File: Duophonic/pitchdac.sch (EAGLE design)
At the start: 30 parts, among them IC1 AD5781ARUZ, U1 opa2186, U2 opa2186

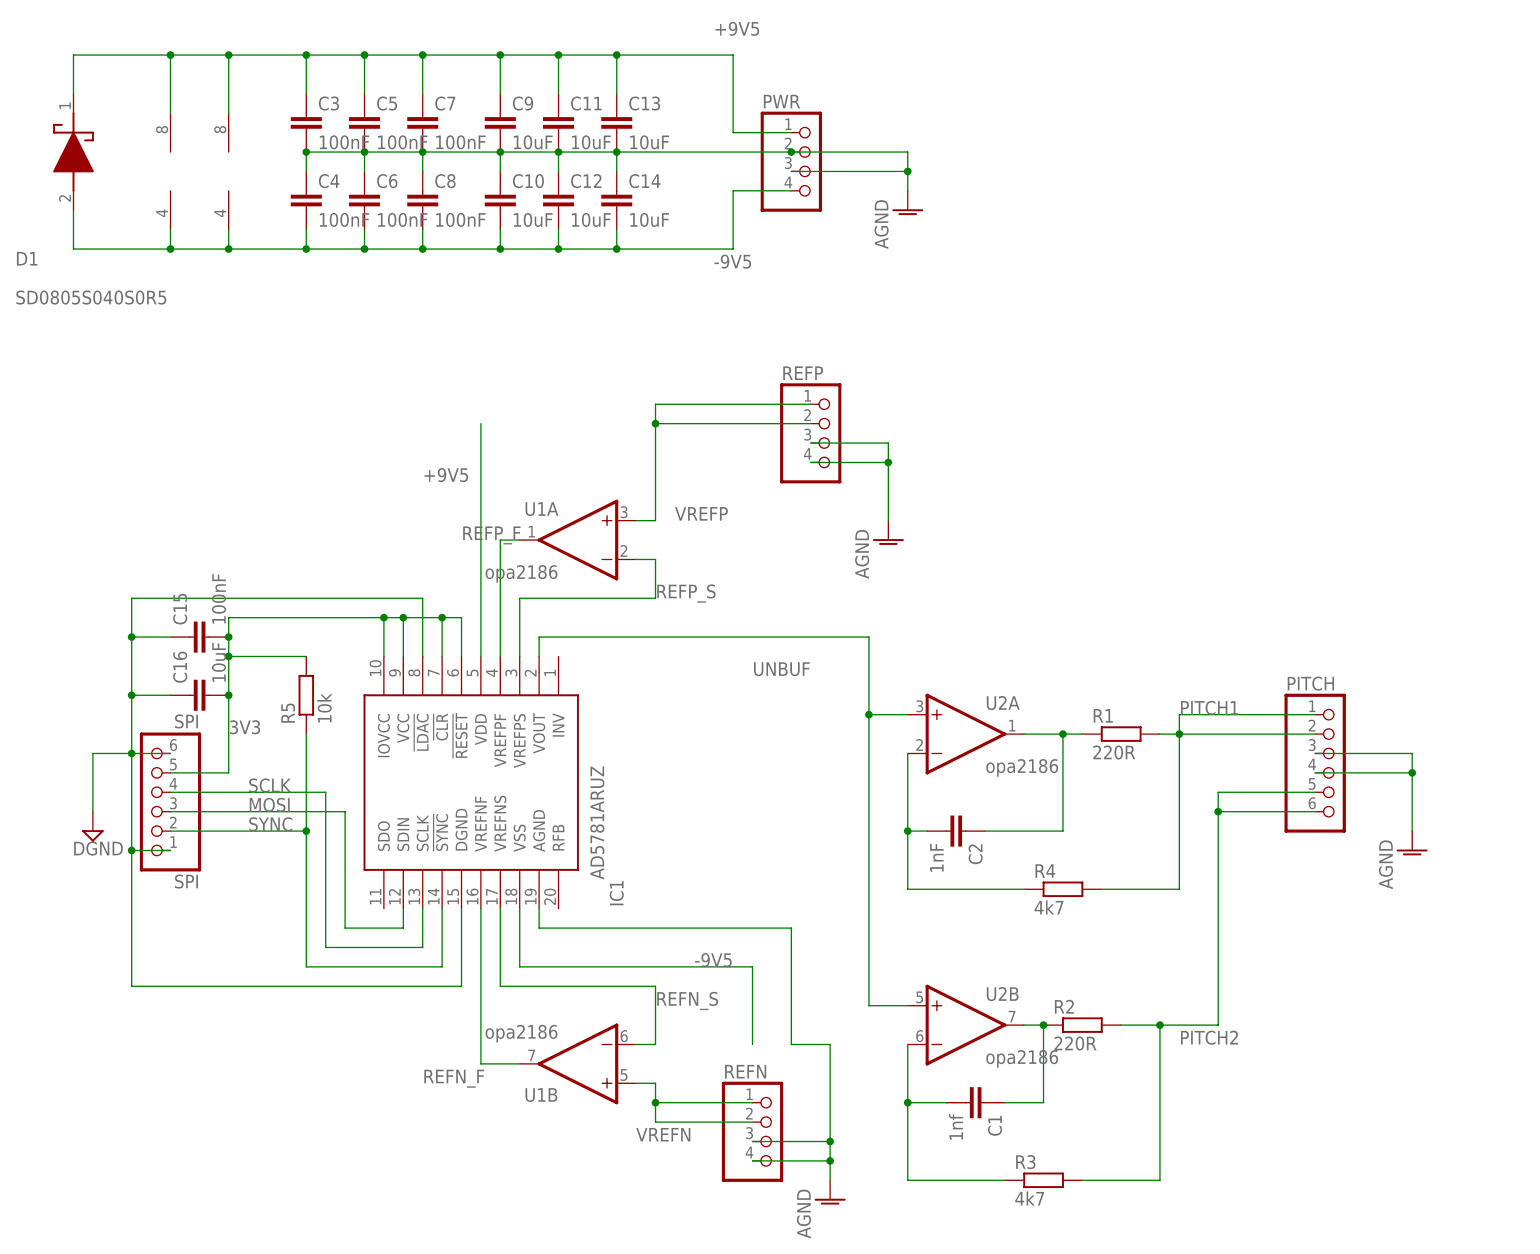
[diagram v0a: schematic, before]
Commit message: correct stupid error
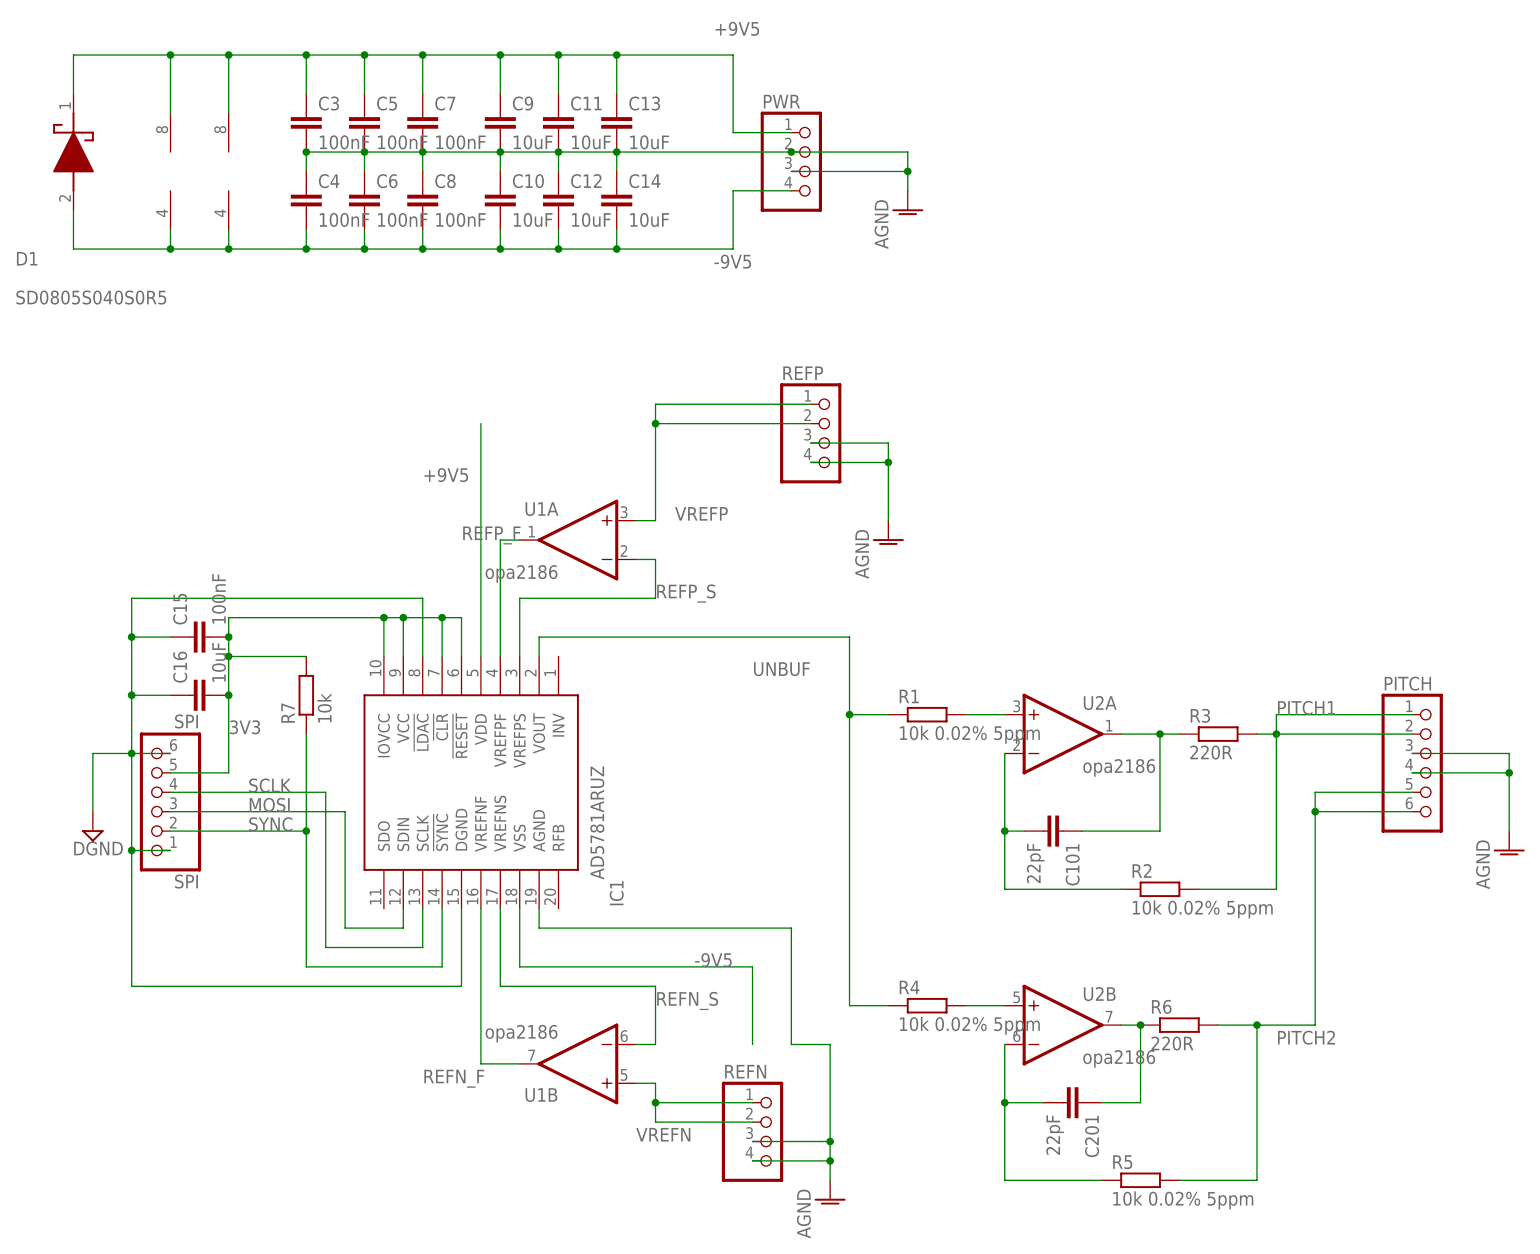
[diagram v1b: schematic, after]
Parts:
- removed C1: 1nf, rcl:C-EUC0805K
- removed C2: 1nF, rcl:C-EUC0805K
- added C101, C201: 22pF, rcl:C-EUC0805K
- added R6: 220R, rcl:R-EU_R0805W
- added R7: 10k, rcl:R-EU_R0805W
- R1, R2: value 220R -> 10k 0.02% 5ppm
- R3: value 4k7 -> 220R
- R4: value 4k7 -> 10k 0.02% 5ppm
- R5: value 10k -> 10k 0.02% 5ppm
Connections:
- new net N$2: R1.2, U2A.+IN
- new net N$3: R4.2, U2B.+IN
- net 3V3: now also R7.2; no longer R5.2
- net N$1: now also C201.2, R5.1; no longer C1.2, R3.1
- net N$15: now also C201.1, R6.1; no longer C1.1, R2.1
- net N$16: now also C101.1, R3.1; no longer C2.1, R1.1
- net N$5: now also C101.2, R2.1; no longer C2.2, R4.1
- net PITCH1: now also R2.2, R3.2; no longer R1.2, R4.2
- net PITCH2: now also R5.2, R6.2; no longer R2.2, R3.2
- net SYNC: now also R7.1; no longer R5.1
- net UNBUF: now also R1.1, R4.1; no longer U2A.+IN, U2B.+IN
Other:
- moved on the sheet: PITCH, R1, R2, R3, R4, R5, U2A, U2B

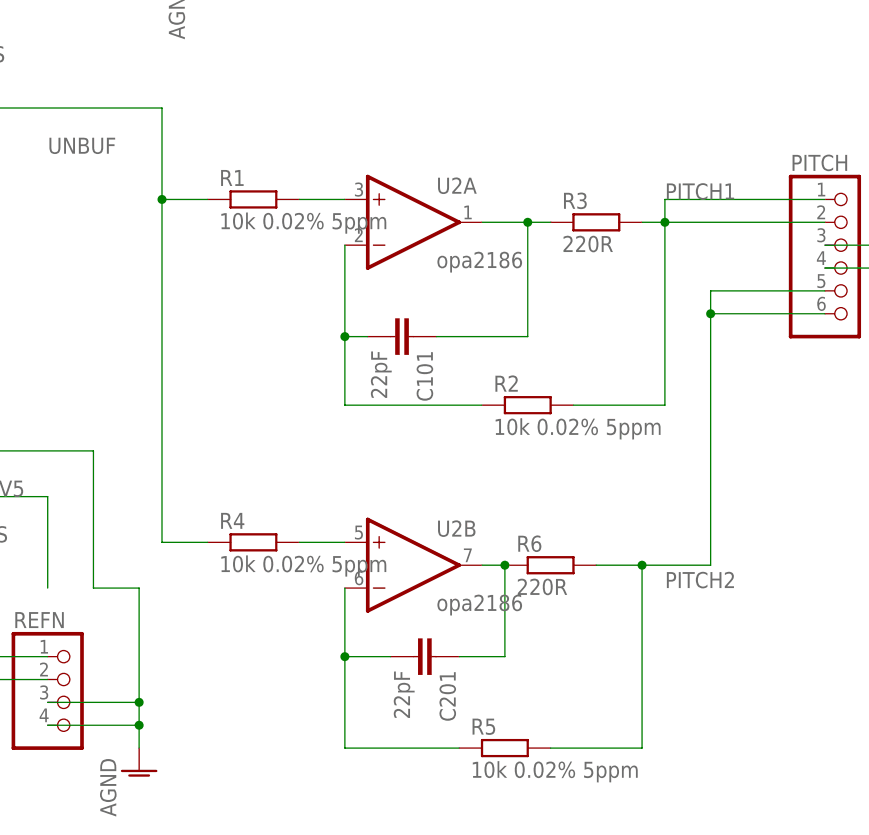
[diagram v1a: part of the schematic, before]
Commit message: idiot!!!
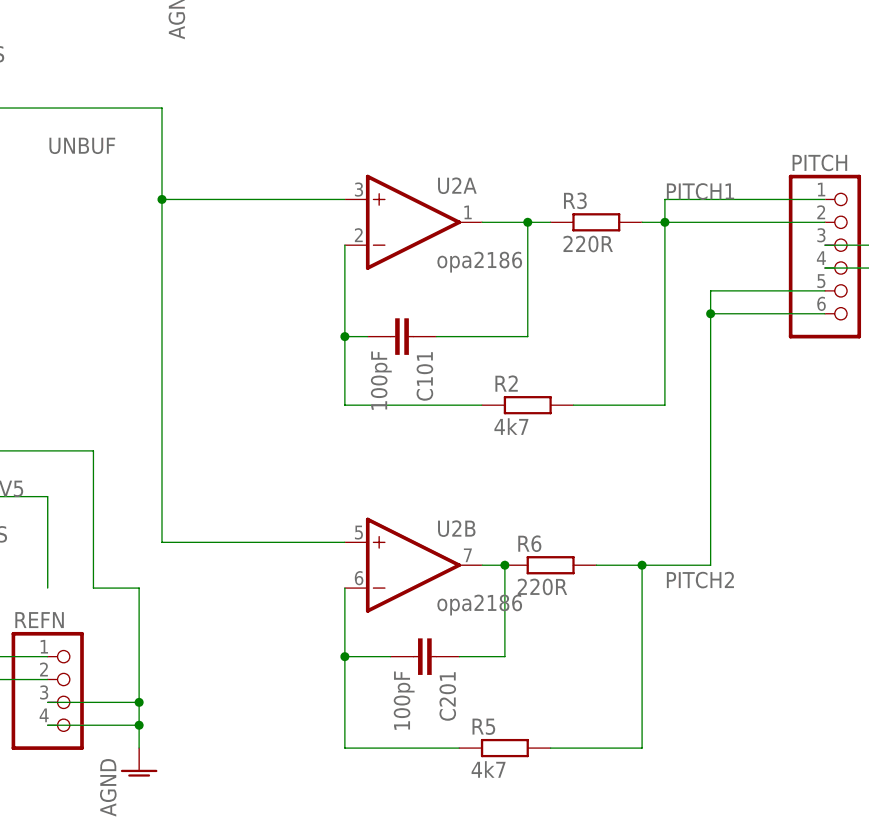
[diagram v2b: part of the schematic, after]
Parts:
- removed R1, R4: 10k 0.02% 5ppm, rcl:R-EU_R0805W
- C101, C201: value 22pF -> 100pF
- R2, R5: value 10k 0.02% 5ppm -> 4k7
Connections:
- removed net N$2: R1.2, U2A.+IN
- removed net N$3: R4.2, U2B.+IN
- net UNBUF: now also U2A.+IN, U2B.+IN; no longer R1.1, R4.1
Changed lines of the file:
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@@
 <part name="AGND3" library="supply1" library_urn="urn:adsk.eagle:library:371" deviceset="AGND" device=""/>
 <part name="AGND4" library="supply1" library_urn="urn:adsk.eagle:library:371" deviceset="AGND" device=""/>
-<part name="C201" library="rcl" library_urn="urn:adsk.eagle:library:334" deviceset="C-EU" device="C0805K" package3d_urn="urn:adsk.eagle:package:23681/2" value="22pF"/>
-<part name="C101" library="rcl" library_urn="urn:adsk.eagle:library:334" deviceset="C-EU" device="C0805K" package3d_urn="urn:adsk.eagle:package:23681/2" value="22pF"/>
+<part name="C201" library="rcl" library_urn="urn:adsk.eagle:library:334" deviceset="C-EU" device="C0805K" package3d_urn="urn:adsk.eagle:package:23681/2" value="100pF"/>
+<part name="C101" library="rcl" library_urn="urn:adsk.eagle:library:334" deviceset="C-EU" device="C0805K" package3d_urn="urn:adsk.eagle:package:23681/2" value="100pF"/>
 <part name="R3" library="rcl" library_urn="urn:adsk.eagle:library:334" deviceset="R-EU_" device="R0805W" package3d_urn="urn:adsk.eagle:package:23537/2" value="220R"/>
 <part name="R6" library="rcl" library_urn="urn:adsk.eagle:library:334" deviceset="R-EU_" device="R0805W" package3d_urn="urn:adsk.eagle:package:23537/2" value="220R"/>
-<part name="R5" library="rcl" library_urn="urn:adsk.eagle:library:334" deviceset="R-EU_" device="R0805W" package3d_urn="urn:adsk.eagle:package:23537/2" value="10k 0.02% 5ppm"/>
-<part name="R2" library="rcl" library_urn="urn:adsk.eagle:library:334" deviceset="R-EU_" device="R0805W" package3d_urn="urn:adsk.eagle:package:23537/2" value="10k 0.02% 5ppm"/>
+<part name="R5" library="rcl" library_urn="urn:adsk.eagle:library:334" deviceset="R-EU_" device="R0805W" package3d_urn="urn:adsk.eagle:package:23537/2" value="4k7"/>
+<part name="R2" library="rcl" library_urn="urn:adsk.eagle:library:334" deviceset="R-EU_" device="R0805W" package3d_urn="urn:adsk.eagle:package:23537/2" value="4k7"/>
 <part name="C3" library="rcl" library_urn="urn:adsk.eagle:library:334" deviceset="C-EU" device="C1206" package3d_urn="urn:adsk.eagle:package:23618/2" value="100nF"/>
 <part name="C4" library="rcl" library_urn="urn:adsk.eagle:library:334" deviceset="C-EU" device="C1206" package3d_urn="urn:adsk.eagle:package:23618/2" value="100nF"/>
@@
 <part name="PITCH" library="pinhead" library_urn="urn:adsk.eagle:library:325" deviceset="PINHD-1X6" device="/90" package3d_urn="urn:adsk.eagle:package:22475/2"/>
 <part name="R7" library="rcl" library_urn="urn:adsk.eagle:library:334" deviceset="R-EU_" device="R0805W" package3d_urn="urn:adsk.eagle:package:23537/2" value="10k"/>
-<part name="R1" library="rcl" library_urn="urn:adsk.eagle:library:334" deviceset="R-EU_" device="R0805W" package3d_urn="urn:adsk.eagle:package:23537/2" value="10k 0.02% 5ppm"/>
-<part name="R4" library="rcl" library_urn="urn:adsk.eagle:library:334" deviceset="R-EU_" device="R0805W" package3d_urn="urn:adsk.eagle:package:23537/2" value="10k 0.02% 5ppm"/>
 </parts>
 <sheets>
@@
 <attribute name="NAME" x="21.3614" y="59.69" size="1.778" layer="95" rot="R90"/>
 <attribute name="VALUE" x="26.162" y="59.69" size="1.778" layer="96" rot="R90"/>
-</instance>
-<instance part="R1" gate="G$1" x="104.14" y="60.96" smashed="yes">
-<attribute name="NAME" x="100.33" y="62.4586" size="1.778" layer="95"/>
-<attribute name="VALUE" x="100.33" y="57.658" size="1.778" layer="96"/>
-</instance>
-<instance part="R4" gate="G$1" x="104.14" y="22.86" smashed="yes">
-<attribute name="NAME" x="100.33" y="24.3586" size="1.778" layer="95"/>
-<attribute name="VALUE" x="100.33" y="19.558" size="1.778" layer="96"/>
 </instance>
 </instances>
@@
 <wire x1="53.34" y1="71.12" x2="93.98" y2="71.12" width="0.1524" layer="91"/>
 <wire x1="93.98" y1="71.12" x2="93.98" y2="60.96" width="0.1524" layer="91"/>
-<pinref part="R4" gate="G$1" pin="1"/>
 <wire x1="93.98" y1="60.96" x2="93.98" y2="22.86" width="0.1524" layer="91"/>
-<wire x1="93.98" y1="22.86" x2="99.06" y2="22.86" width="0.1524" layer="91"/>
-<pinref part="R1" gate="G$1" pin="1"/>
-<wire x1="99.06" y1="60.96" x2="93.98" y2="60.96" width="0.1524" layer="91"/>
 <junction x="93.98" y="60.96"/>
+<pinref part="U2" gate="A" pin="+IN"/>
+<wire x1="114.3" y1="60.96" x2="93.98" y2="60.96" width="0.1524" layer="91"/>
+<pinref part="U2" gate="B" pin="+IN"/>
+<wire x1="114.3" y1="22.86" x2="93.98" y2="22.86" width="0.1524" layer="91"/>
 </segment>
 </net>
@@
 </segment>
 </net>
-<net name="N$2" class="0">
-<segment>
-<pinref part="U2" gate="A" pin="+IN"/>
-<wire x1="109.22" y1="60.96" x2="114.3" y2="60.96" width="0.1524" layer="91"/>
-<pinref part="R1" gate="G$1" pin="2"/>
-</segment>
-</net>
-<net name="N$3" class="0">
-<segment>
-<pinref part="U2" gate="B" pin="+IN"/>
-<wire x1="109.22" y1="22.86" x2="114.3" y2="22.86" width="0.1524" layer="91"/>
-<pinref part="R4" gate="G$1" pin="2"/>
-</segment>
-</net>
